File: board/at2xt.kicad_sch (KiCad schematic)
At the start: 15 parts, among them J1 Conn_01x04, J2 XT, J3 AT, J4 PS/2, U1 MCP1700-3302E_TO92, U2 MSP430G2211IPW14

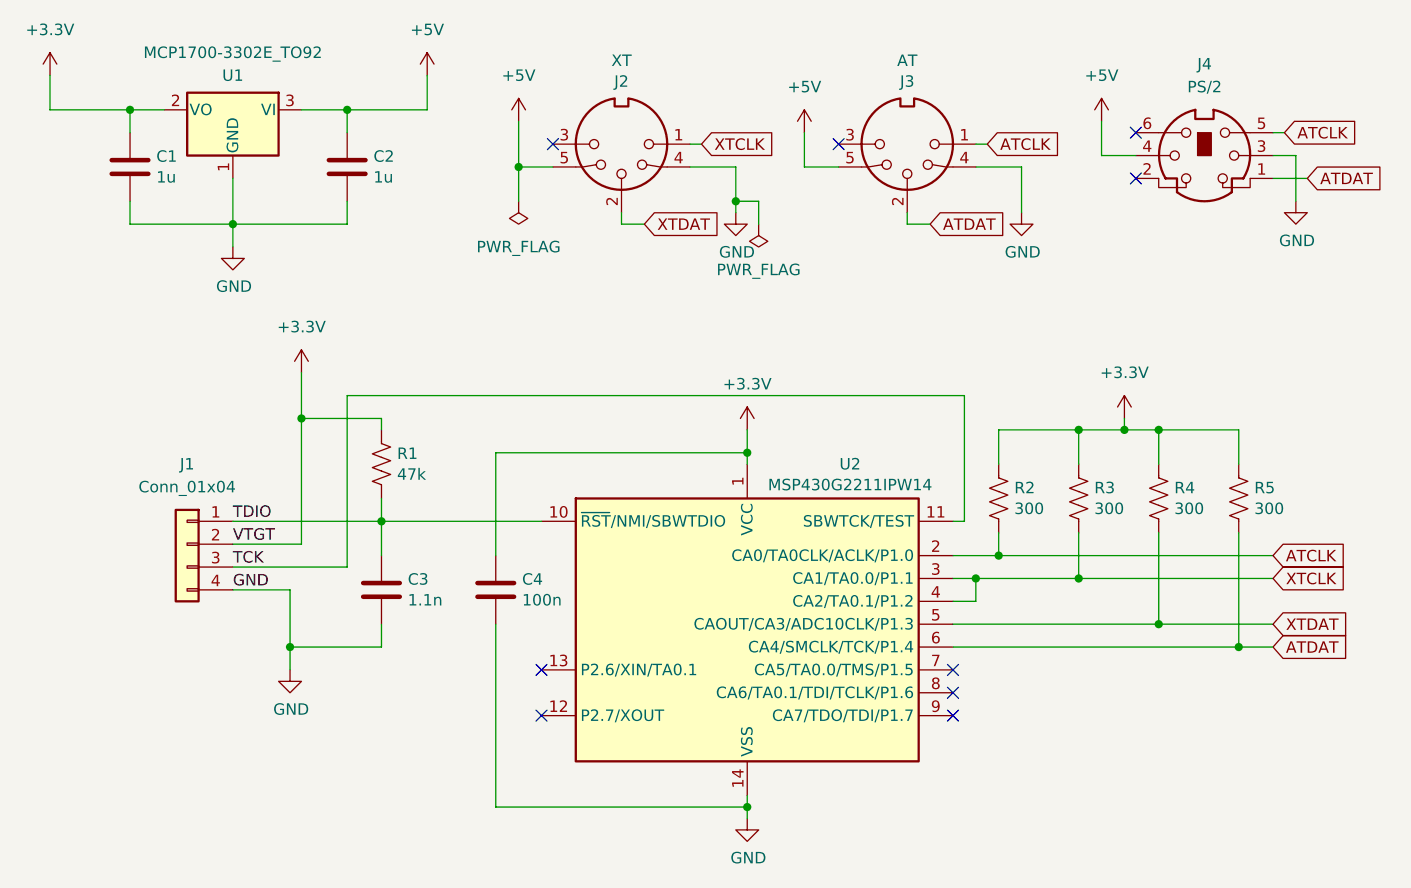
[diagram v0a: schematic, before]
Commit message: Apply some suggestions from dragonmux's hoard.
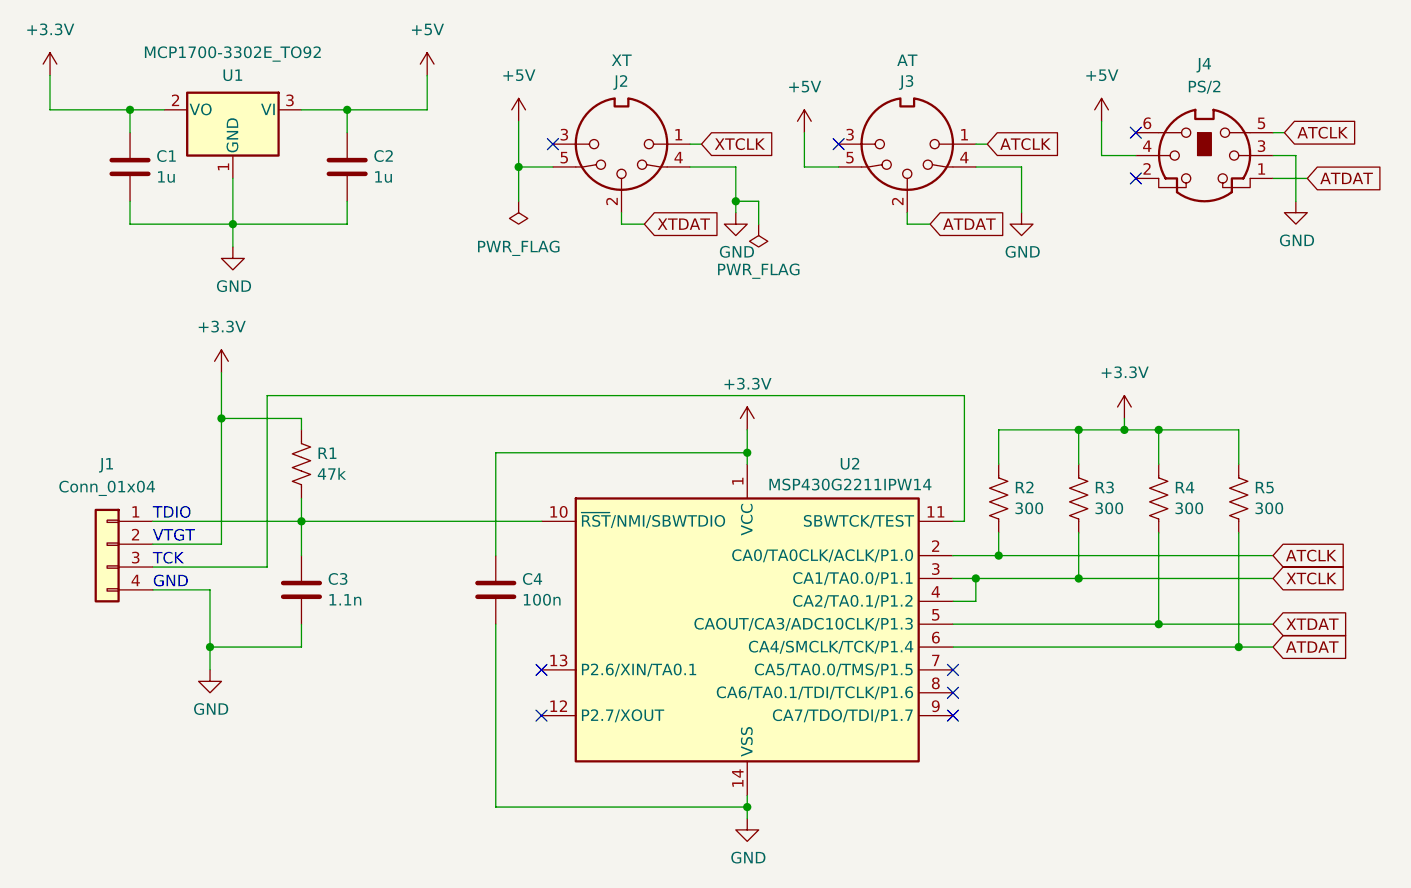
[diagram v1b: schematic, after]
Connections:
- net TCK: no longer names the net of J1.3 (Pin_3), U2.11 (SBWTCK/TEST)
- net TDIO: no longer names the net of C3.1, J1.1 (Pin_1), R1.2, U2.10 (~{RST}/NMI/SBWTDIO)
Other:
- note added: "GND"
- note added: "TCK"
- note added: "TDIO"
- note added: "VTGT"
- moved on the sheet: C3, J1, R1
